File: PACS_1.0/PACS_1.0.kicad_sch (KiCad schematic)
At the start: 8 parts, among them U1 MSP430G2553IN20

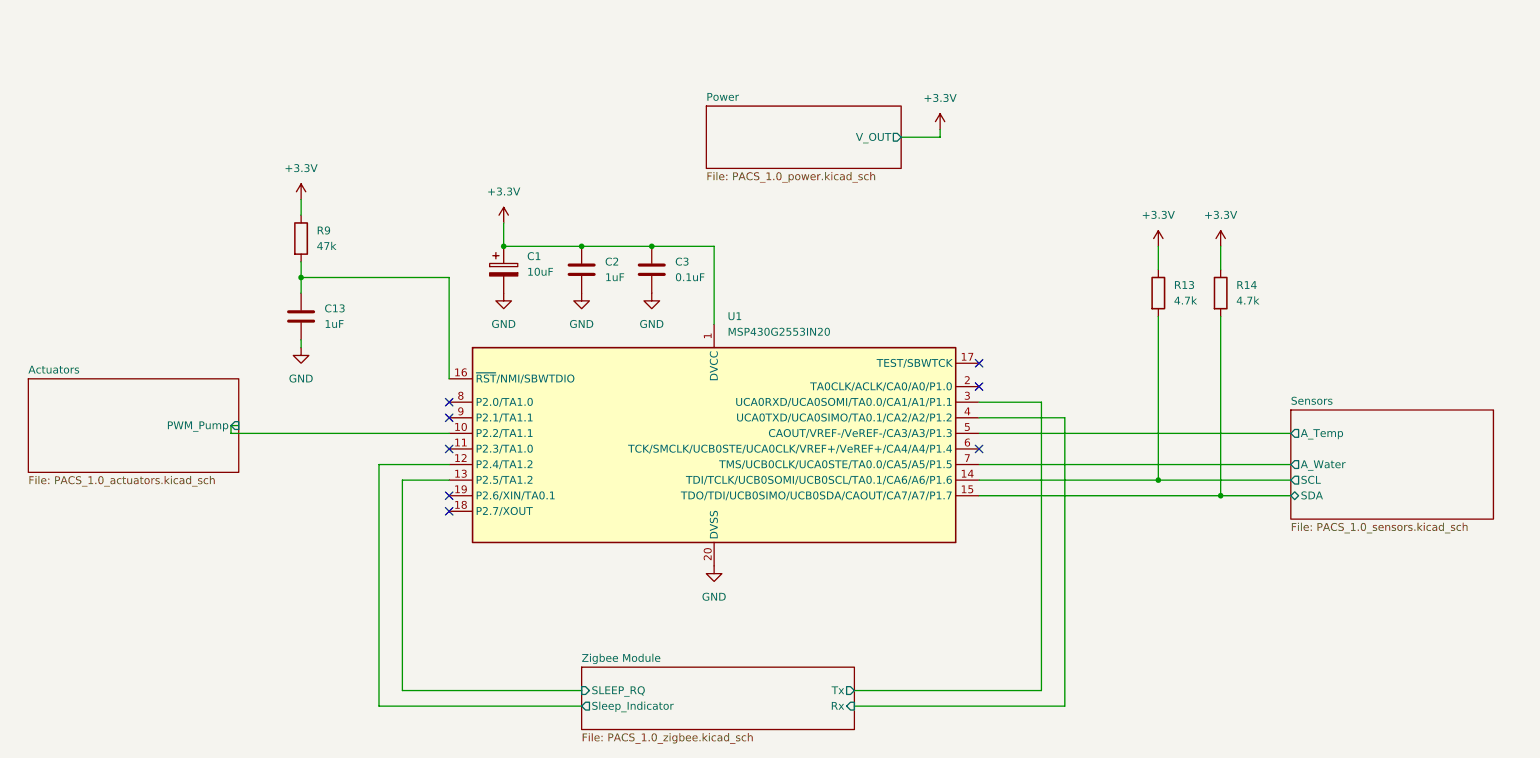
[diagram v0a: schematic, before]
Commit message: COMPLETE PACS v1.0
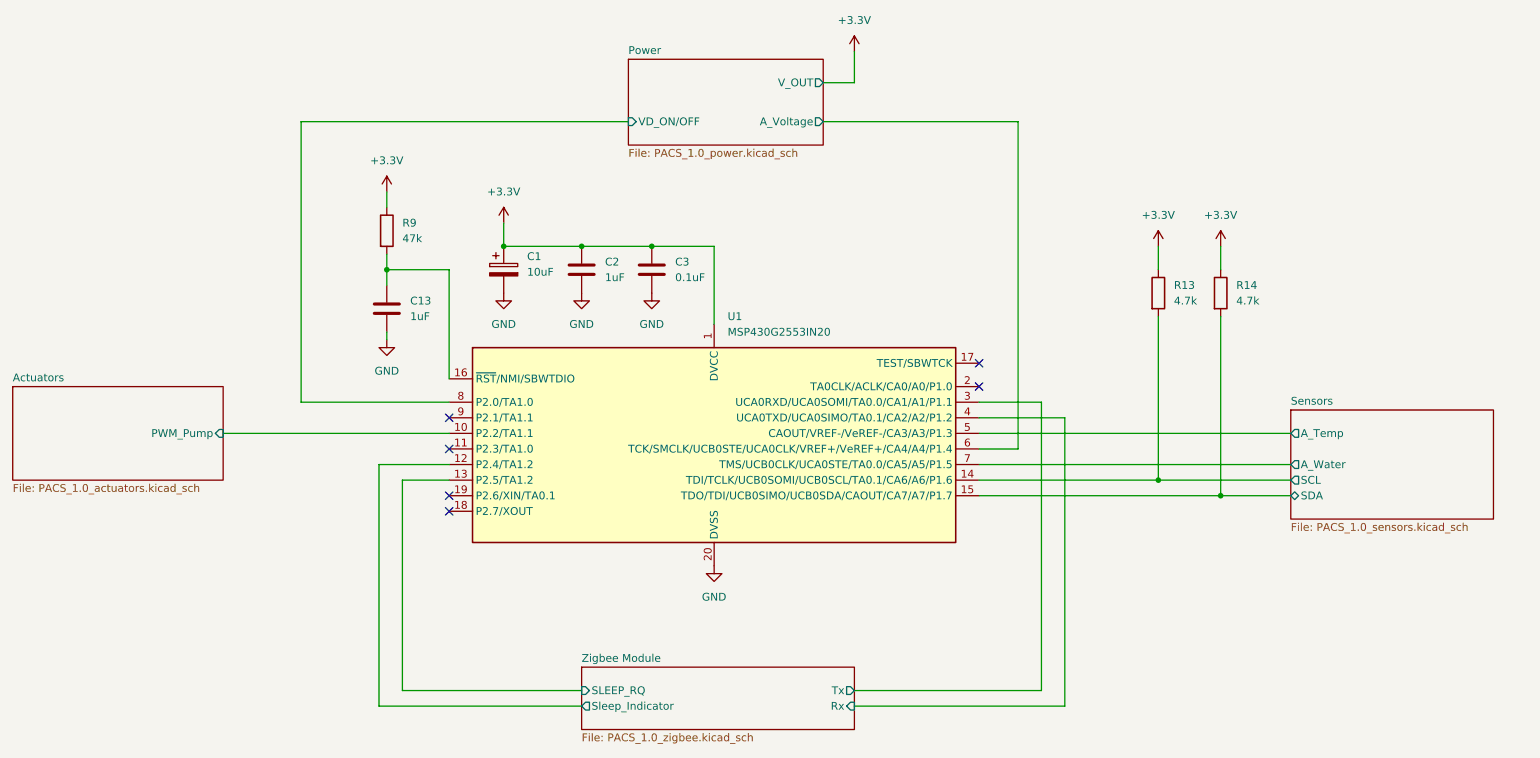
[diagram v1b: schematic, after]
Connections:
- net Power/A_Voltage: now reaches U1.6 (TCK/SMCLK/UCB0STE/UCA0CLK/VREF+/VeREF+/CA4/A4/P1.4)
- net Power/VD_ON/OFF: now reaches U1.8 (P2.0/TA1.0)
- no-connect marks 8 -> 6
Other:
- sheet Power ports: added A_Voltage, VD_ON/OFF; removed none
- moved on the sheet: C13, R9
